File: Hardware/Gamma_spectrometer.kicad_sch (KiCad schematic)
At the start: 47 parts, among them J1 Conn_01x04, J10 Test Pad, J11 Test Pad, J12 Test Pad, J2 Conn_01x04, J3 Conn_01x01, J4 Conn_01x04, J5 Test Pad, J6 Test Pad, J7 Test Pad, J8 Test Pad, J9 Test Pad, Q1 2N7002, U11 ATtiny1616-M, U2 LM317L_SO8, U3 OPA356xxDBV, U4 OPA357AIDVBR, U5 OPA357AIDVBR, U6 LMV7219M7, U7 OPA356xxDBV, U8 FODM217A

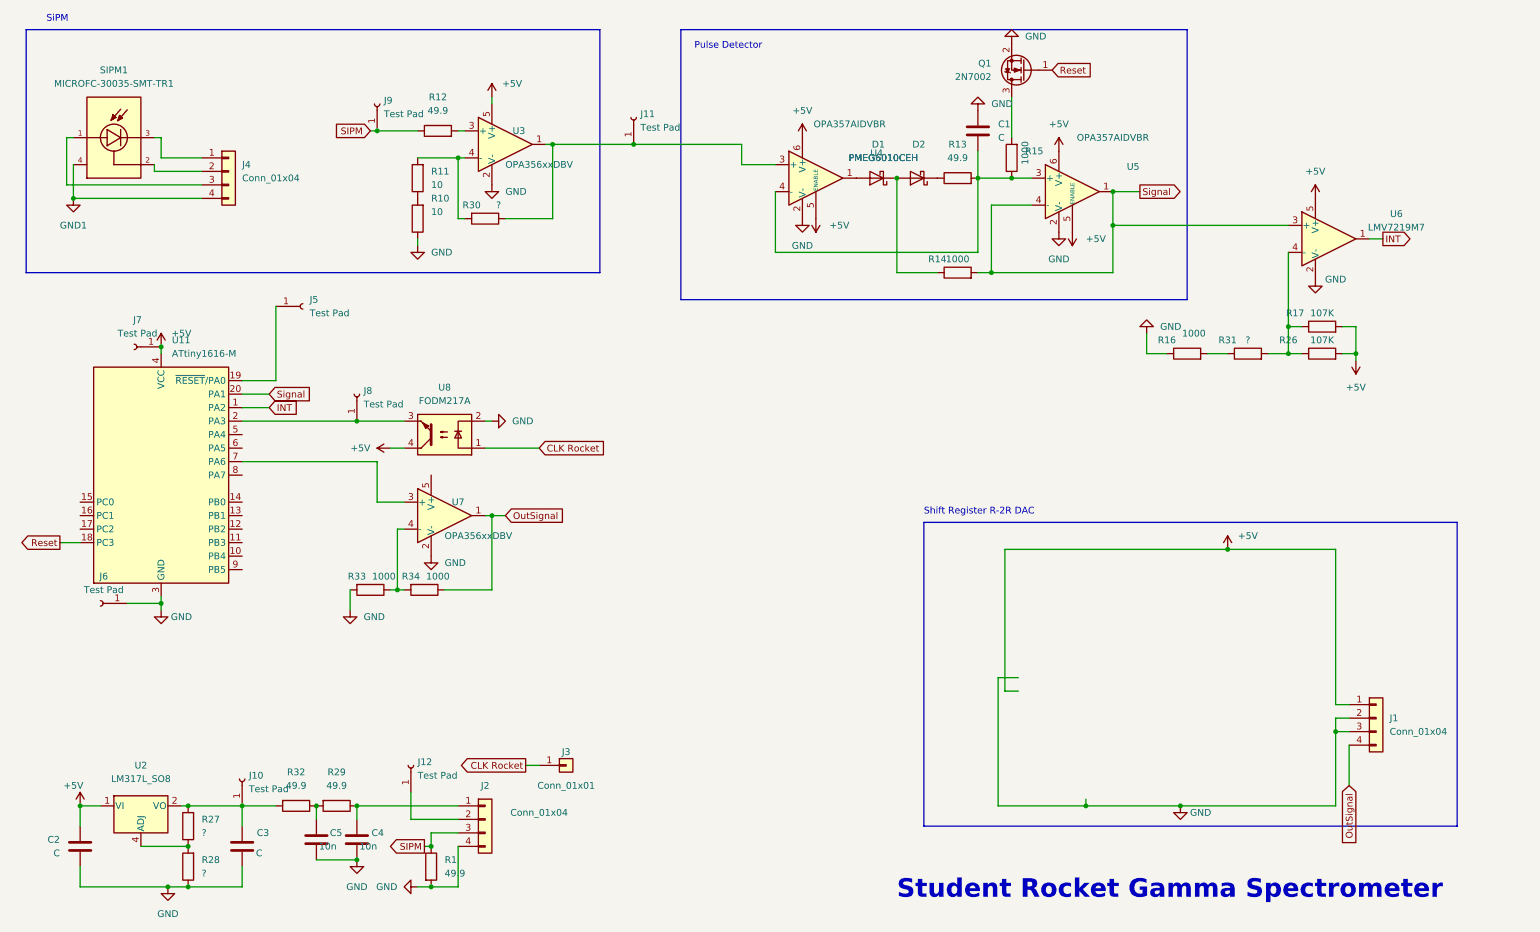
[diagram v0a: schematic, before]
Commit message: fixed som BOM stuff
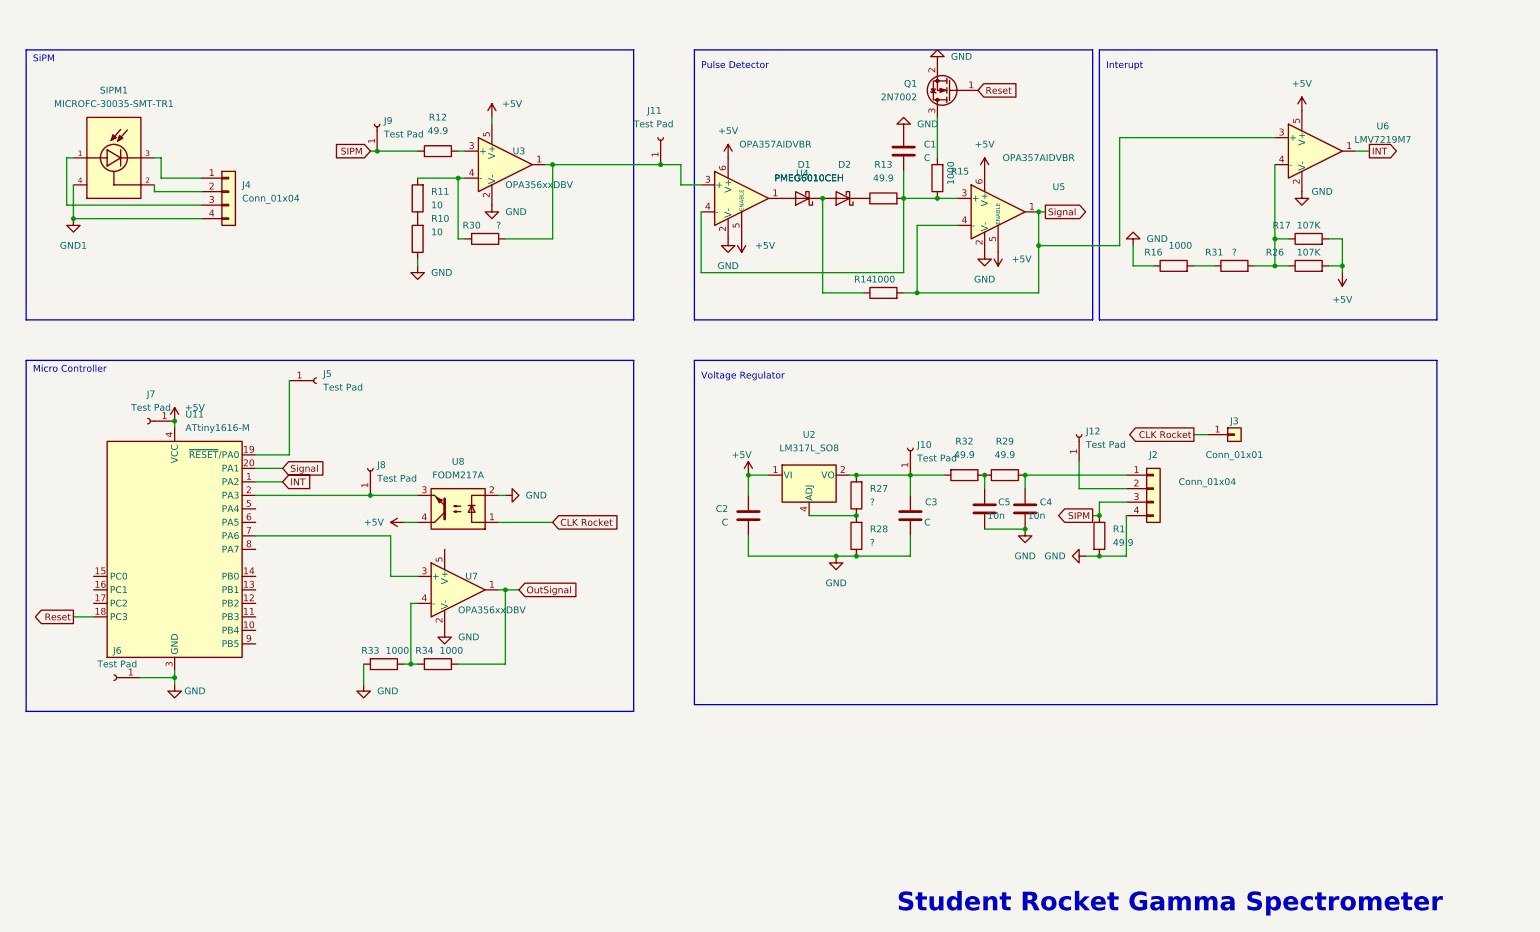
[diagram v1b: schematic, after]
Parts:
- removed J1: Conn_01x04, Connector_PinHeader_2.00mm:PinHeader_1x04_P2.00mm_Vertical, symbol Connector_Generic:Conn_01x04
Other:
- note added: "Interupt"
- note added: "Micro Controller"
- note added: "Voltage Regulator"
- note removed: "Shift Register R-2R DAC"
- moved on the sheet: C1, C2, C3, C4, C5, D1, D2, J10, J11, J12, J2, J3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
